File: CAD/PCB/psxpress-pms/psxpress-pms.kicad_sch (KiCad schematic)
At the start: 40 parts, among them IC1 BQ25606RGER, IC2 MAX16054AZT+T, IC3 TPS61023DRLT, IC4 TPS564255DRLR, Q1 AO3401A, SW1 SW_SPST

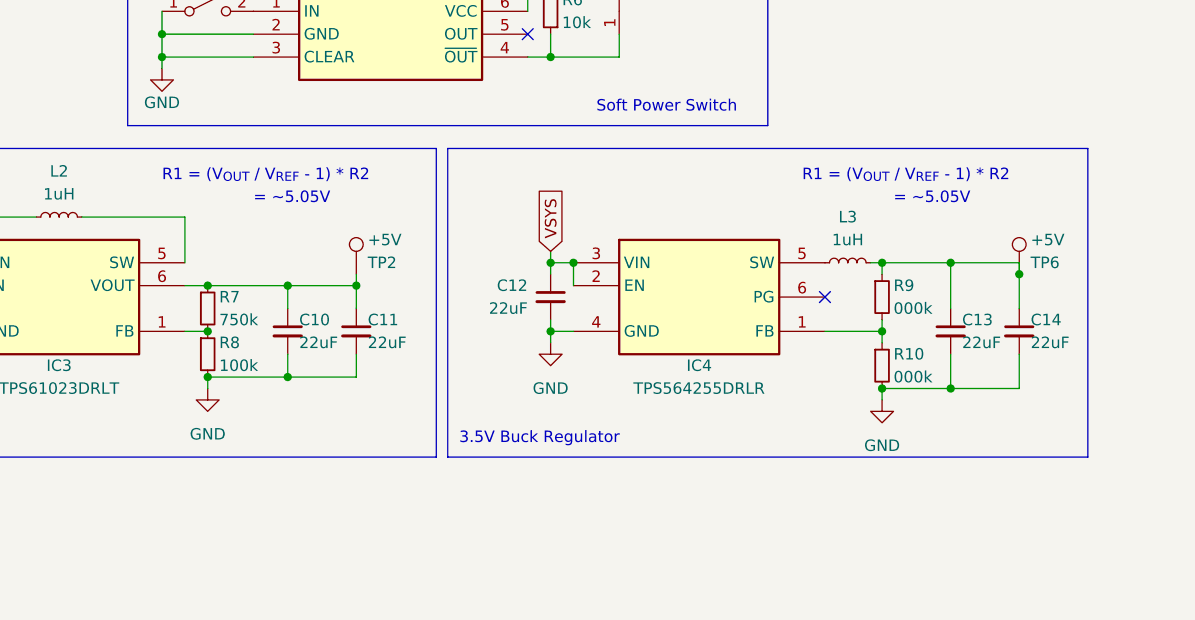
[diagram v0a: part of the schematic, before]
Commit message: pms - forgot to save again
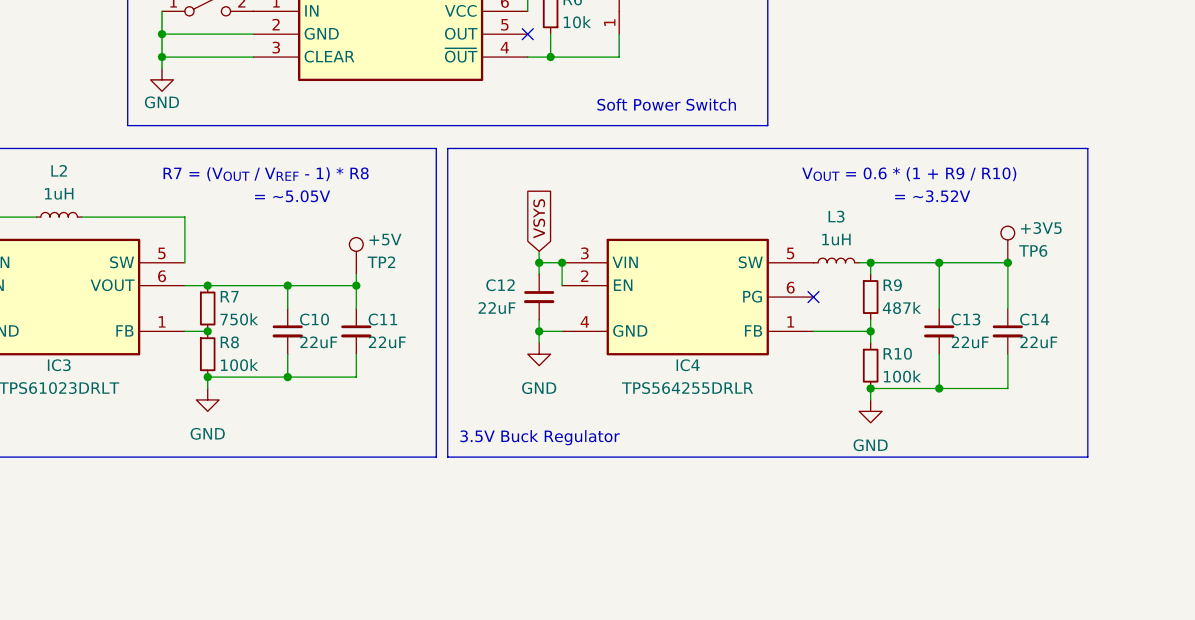
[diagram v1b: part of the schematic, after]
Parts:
- R10: value 000k -> 100k
- R9: value 000k -> 487k
- TP6: value +5V -> +3V5
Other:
- note added: "= ~3.52V"
- note added: "R7 = (V_{OUT} / V_{REF} - 1) * R8"
- note added: "V_{OUT} = 0.6 * (1 + R9 / R10)"
- note removed: "R1 = (V_{OUT} / V_{REF} - 1) * R2"
- moved on the sheet: C12, C13, C14, IC4, L3, R10, R9, TP6
